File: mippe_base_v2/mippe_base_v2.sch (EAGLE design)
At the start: 21 parts, among them J9 BURNIN, SW1 BTN-PTS810, U1 ATMEGA328P-AUR, Y1 16MHz

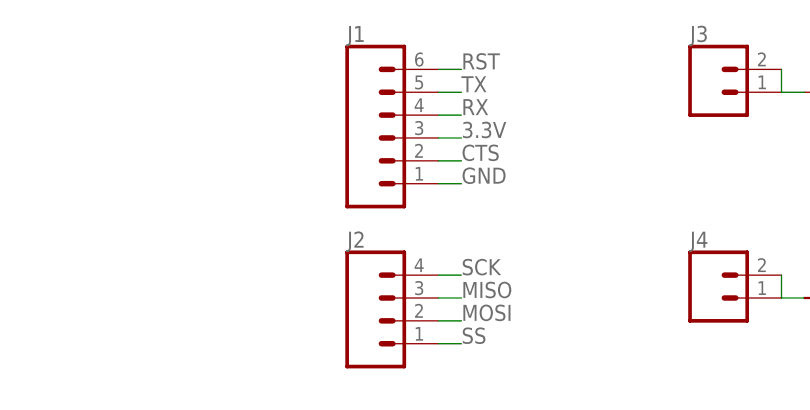
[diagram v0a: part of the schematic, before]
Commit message: fix rst and flip conn
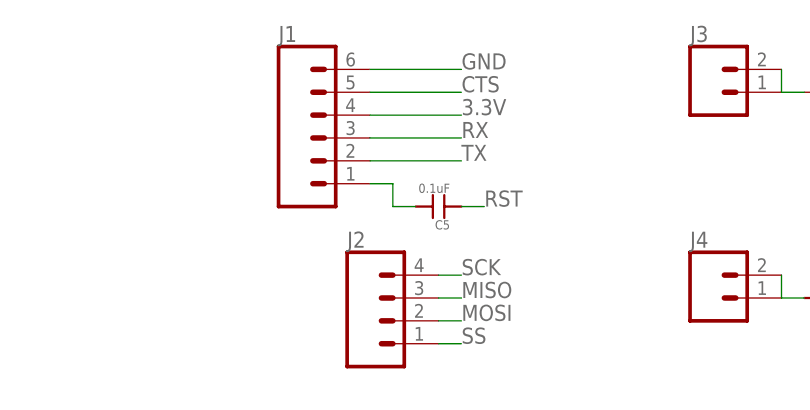
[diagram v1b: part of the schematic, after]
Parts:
- added C5: 0.1uF, scono:CAP0603-CAP
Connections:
- new net N$3: C5.2, J1.1
- net 3.3V: now also J1.4; no longer J1.3
- net CTS: now also J1.5; no longer J1.2
- net GND: now also J1.6; no longer J1.1
- net RST: now also C5.1; no longer J1.6
- net RX: now also J1.3; no longer J1.4
- net TX: now also J1.2; no longer J1.5
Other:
- moved on the sheet: J1
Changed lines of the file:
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@@
 <part name="FRAME1" library="scono" deviceset="FRAME_SCHEMATIC" device="">
 <attribute name="AUTHOR" value="S. Ono"/>
-<attribute name="REV" value="A"/>
+<attribute name="REV" value="C"/>
 <attribute name="SUBSYSTEM_NAME" value="mippe_base"/>
 </part>
@@
 <part name="U$9" library="scono" deviceset="3.3V" device=""/>
 <part name="SUPPLY2" library="scono" deviceset="GND" device=""/>
+<part name="C5" library="scono" deviceset="CAP" device="0603-CAP" value="0.1uF"/>
 </parts>
 <sheets>
@@
 <attribute name="VALUE" x="12.7" y="107.95" size="1.016" layer="96" rot="R270"/>
 </instance>
-<instance part="J1" gate="G$1" x="172.72" y="157.48" smashed="yes">
-<attribute name="VALUE" x="167.64" y="147.574" size="1.778" layer="96" font="vector"/>
-<attribute name="NAME" x="167.64" y="168.148" size="1.778" layer="95" font="vector"/>
+<instance part="J1" gate="G$1" x="165.1" y="157.48" smashed="yes">
+<attribute name="VALUE" x="160.02" y="147.574" size="1.778" layer="96" font="vector"/>
+<attribute name="NAME" x="160.02" y="168.148" size="1.778" layer="95" font="vector"/>
 </instance>
 <instance part="J2" gate="G$1" x="172.72" y="137.16" smashed="yes">
@@
 <instance part="SUPPLY2" gate="GND" x="137.16" y="50.8" smashed="yes" rot="R90">
 <attribute name="VALUE" x="139.7" y="49.53" size="1.016" layer="96" rot="R90"/>
+</instance>
+<instance part="C5" gate="G$1" x="177.8" y="149.86" smashed="yes" rot="R180">
+<attribute name="NAME" x="179.07" y="148.336" size="1.016" layer="95" rot="R180"/>
+<attribute name="VALUE" x="179.07" y="152.4" size="1.016" layer="96" rot="R180"/>
 </instance>
 </instances>
@@
 </segment>
 <segment>
-<pinref part="J1" gate="G$1" pin="1"/>
-<wire x1="177.8" y1="152.4" x2="180.34" y2="152.4" width="0.1524" layer="91"/>
-<label x="180.34" y="152.4" size="1.778" layer="95"/>
-</segment>
-<segment>
 <pinref part="D2" gate="G$1" pin="C"/>
 <pinref part="SUPPLY10" gate="GND" pin="GND"/>
@@
 <pinref part="U1" gate="G$1" pin="GND"/>
 <pinref part="SUPPLY2" gate="GND" pin="GND"/>
+</segment>
+<segment>
+<pinref part="J1" gate="G$1" pin="6"/>
+<wire x1="170.18" y1="165.1" x2="180.34" y2="165.1" width="0.1524" layer="91"/>
+<label x="180.34" y="165.1" size="1.778" layer="95"/>
 </segment>
 </net>
@@
 <wire x1="215.9" y1="162.56" x2="218.44" y2="162.56" width="0.1524" layer="91"/>
 <pinref part="U$6" gate="G$1" pin="3.3V"/>
-</segment>
-<segment>
-<pinref part="J1" gate="G$1" pin="3"/>
-<wire x1="177.8" y1="157.48" x2="180.34" y2="157.48" width="0.1524" layer="91"/>
-<label x="180.34" y="157.48" size="1.778" layer="95"/>
 </segment>
 <segment>
@@
 <wire x1="134.62" y1="109.22" x2="134.62" y2="106.68" width="0.1524" layer="91"/>
 </segment>
+<segment>
+<pinref part="J1" gate="G$1" pin="4"/>
+<wire x1="170.18" y1="160.02" x2="180.34" y2="160.02" width="0.1524" layer="91"/>
+<label x="180.34" y="160.02" size="1.778" layer="95"/>
+</segment>
 </net>
 <net name="SCL" class="0">
@@
 <net name="RX" class="0">
 <segment>
-<pinref part="J1" gate="G$1" pin="4"/>
-<wire x1="177.8" y1="160.02" x2="180.34" y2="160.02" width="0.1524" layer="91"/>
-<label x="180.34" y="160.02" size="1.778" layer="95"/>
-</segment>
-<segment>
 <pinref part="J7" gate="G$1" pin="1"/>
 <wire x1="215.9" y1="104.14" x2="218.44" y2="104.14" width="0.1524" layer="91"/>
@@
 <label x="139.7" y="93.98" size="1.778" layer="95"/>
 </segment>
+<segment>
+<pinref part="J1" gate="G$1" pin="3"/>
+<wire x1="170.18" y1="157.48" x2="180.34" y2="157.48" width="0.1524" layer="91"/>
+<label x="180.34" y="157.48" size="1.778" layer="95"/>
+</segment>
 </net>
 <net name="TX" class="0">
-<segment>
-<pinref part="J1" gate="G$1" pin="5"/>
-<wire x1="177.8" y1="162.56" x2="180.34" y2="162.56" width="0.1524" layer="91"/>
-<label x="180.34" y="162.56" size="1.778" layer="95"/>
-</segment>
 <segment>
 <pinref part="J7" gate="G$1" pin="2"/>
@@
 <wire x1="134.62" y1="91.44" x2="137.16" y2="91.44" width="0.1524" layer="91"/>
 <label x="139.7" y="91.44" size="1.778" layer="95"/>
+</segment>
+<segment>
+<pinref part="J1" gate="G$1" pin="2"/>
+<wire x1="170.18" y1="154.94" x2="180.34" y2="154.94" width="0.1524" layer="91"/>
+<label x="180.34" y="154.94" size="1.778" layer="95"/>
 </segment>
 </net>
@@
 </segment>
 <segment>
-<pinref part="J1" gate="G$1" pin="6"/>
-<wire x1="177.8" y1="165.1" x2="180.34" y2="165.1" width="0.1524" layer="91"/>
-<label x="180.34" y="165.1" size="1.778" layer="95"/>
-</segment>
-<segment>
 <pinref part="U1" gate="G$1" pin="PC6(!RESET!/PCINT14)"/>
 <wire x1="63.5" y1="55.88" x2="60.96" y2="55.88" width="0.1524" layer="91"/>
@@
 <label x="30.48" y="152.4" size="1.778" layer="95"/>
 </segment>
-</net>
-<net name="CTS" class="0">
-<segment>
-<pinref part="J1" gate="G$1" pin="2"/>
-<wire x1="177.8" y1="154.94" x2="180.34" y2="154.94" width="0.1524" layer="91"/>
-<label x="180.34" y="154.94" size="1.778" layer="95"/>
+<segment>
+<pinref part="C5" gate="G$1" pin="1"/>
+<wire x1="180.34" y1="149.86" x2="182.88" y2="149.86" width="0.1524" layer="91"/>
+<label x="182.88" y="149.86" size="1.778" layer="95"/>
 </segment>
 </net>
@@
 </segment>
 </net>
+<net name="CTS" class="0">
+<segment>
+<pinref part="J1" gate="G$1" pin="5"/>
+<wire x1="170.18" y1="162.56" x2="180.34" y2="162.56" width="0.1524" layer="91"/>
+<label x="180.34" y="162.56" size="1.778" layer="95"/>
+</segment>
+</net>
+<net name="N$3" class="0">
+<segment>
+<pinref part="J1" gate="G$1" pin="1"/>
+<wire x1="170.18" y1="152.4" x2="172.72" y2="152.4" width="0.1524" layer="91"/>
+<wire x1="172.72" y1="152.4" x2="172.72" y2="149.86" width="0.1524" layer="91"/>
+<wire x1="172.72" y1="149.86" x2="175.26" y2="149.86" width="0.1524" layer="91"/>
+<pinref part="C5" gate="G$1" pin="2"/>
+</segment>
+</net>
